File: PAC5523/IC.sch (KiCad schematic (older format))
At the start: 18 parts, among them U11 ENCODER B, U2 ACT4088, U3 MAX3051, U5 ENCODER A, U6 RS485, U7 USBLC6-4, U8 USBLC6-4, U9 USBLC6-4

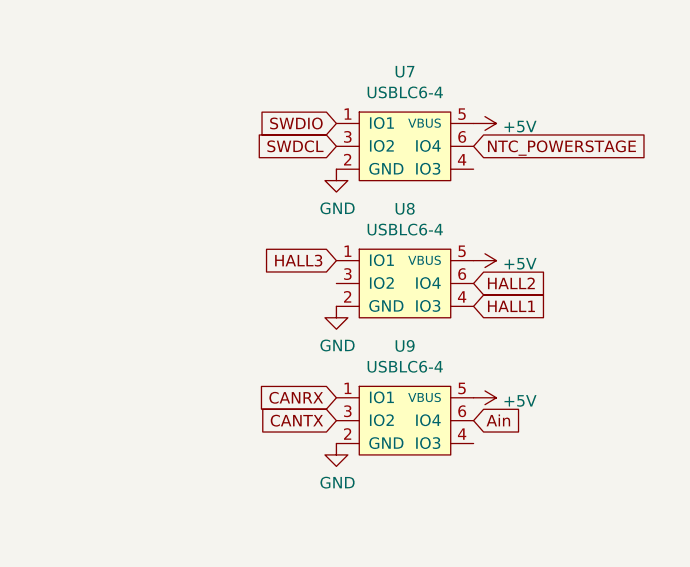
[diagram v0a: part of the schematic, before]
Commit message: finalized board, silkscreen needs some work
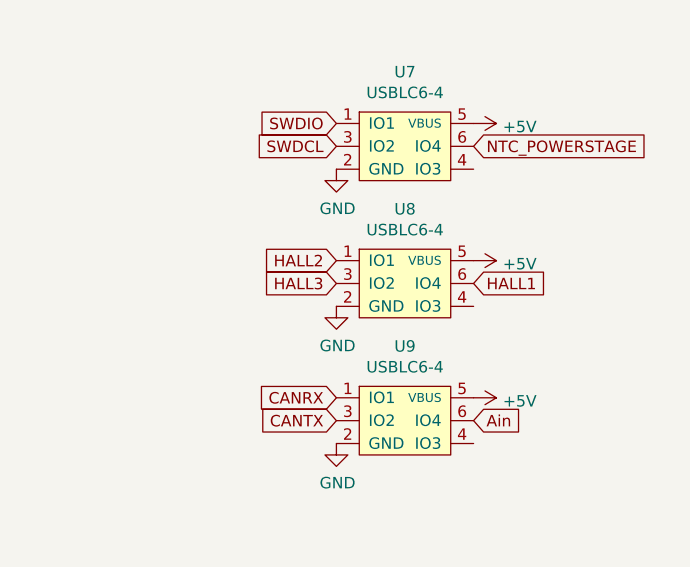
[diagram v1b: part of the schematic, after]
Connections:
- net HALL1: now also U8.6 (IO4); no longer U8.4 (IO3)
- net HALL2: now also U8.1 (IO1); no longer U8.6 (IO4)
- net HALL3: now also U8.3 (IO2); no longer U8.1 (IO1)
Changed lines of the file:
@@
 	1    0    0    -1
 $EndComp
+Text GLabel 8950 3950 0    50   Input ~ 0
+HALL3
 Text GLabel 8950 3850 0    50   Input ~ 0
-HALL3
+HALL2
 Text GLabel 9550 3950 2    50   Input ~ 0
-HALL2
-Text GLabel 9550 4050 2    50   Input ~ 0
 HALL1
 $Comp

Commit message: finalized silkscreen, generated gerber
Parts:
- removed C35, C36, C38: 100n, Capacitor_SMD:C_0603_1608Metric, symbol Device:C_Small
- removed C37: 10u, Capacitor_SMD:C_1206_3216Metric, symbol Device:C_Small
- removed D17: SS310, Diode_SMD:D_SOD-123F, symbol Device:D_Small
- removed D20: SK6812MINI, LED_SMD:LED_SK6812MINI_PLCC4_3.5x3.5mm_P1.75mm, symbol LED:SK6812MINI
- removed L1: 4u7, Inductor_SMD:L_Taiyo-Yuden_MD-4040, symbol Device:L_Small
- removed R40: 4k3, Resistor_SMD:R_0603_1608Metric, symbol Device:R_Small
- removed R41: 100k, Resistor_SMD:R_0603_1608Metric, symbol Device:R_Small
- removed R42: 19k3, Resistor_SMD:R_0603_1608Metric, symbol Device:R_Small
- removed U11: ENCODER B, Package_SO:SOIC-8_3.9x4.9mm_P1.27mm, symbol otter:RS485
- removed U2: ACT4088, Package_TO_SOT_SMD:SOT-23-6, symbol otter:ACT4088
- removed U3: MAX3051, Package_SO:SOIC-8_3.9x4.9mm_P1.27mm, symbol Interface_UART:MAX3051
- removed U5: ENCODER A, Package_SO:SOIC-8_3.9x4.9mm_P1.27mm, symbol otter:RS485
- removed U6: RS485, Package_SO:SOIC-8_3.9x4.9mm_P1.27mm, symbol otter:RS485
- removed U7, U8, U9: USBLC6-4, Package_TO_SOT_SMD:SOT-23-6, symbol otter:USBLC6-4
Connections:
- no-connect marks 1 -> 0
